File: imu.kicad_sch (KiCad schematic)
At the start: 4 parts, among them U8 MC3479

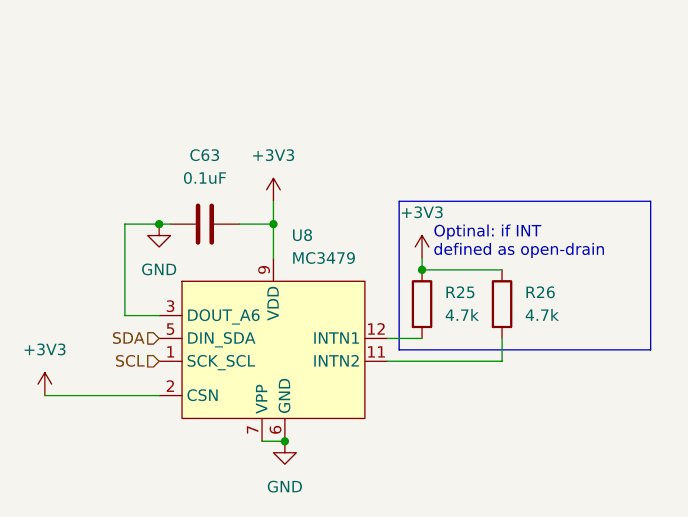
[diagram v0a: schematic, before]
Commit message: schematic creation
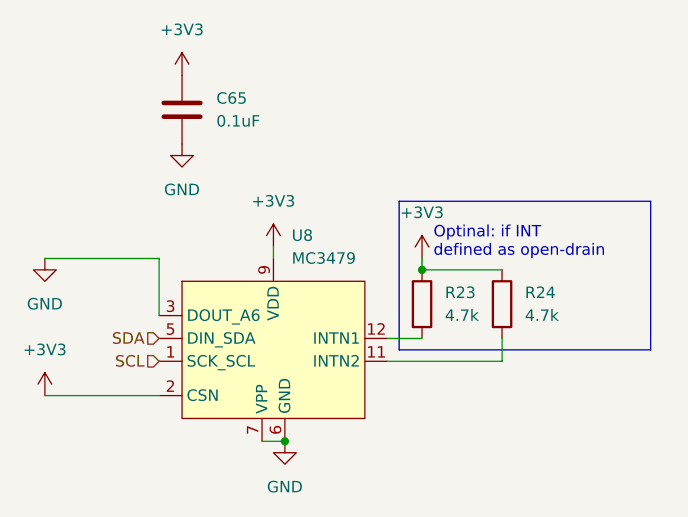
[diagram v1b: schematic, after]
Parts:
- renumbered C63 to C65, R25 to R23, R26 to R24
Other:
- moved on the sheet: C65
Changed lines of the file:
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@@
   (junction (at 157.48 88.9) (diameter 0) (color 0 0 0 0)
   )
-  (junction (at 140.97 83.82) (diameter 0) (color 0 0 0 0)
-  )
-  (junction (at 128.27 83.82) (diameter 0) (color 0 0 0 0)
-  )
   (junction (at 142.24 107.95) (diameter 0) (color 0 0 0 0)
   )
-  (wire (pts (xy 140.97 83.82) (xy 140.97 87.63))
-    (stroke (width 0) (type default) (color 0 0 0 0))
-  )
-  (wire (pts (xy 137.16 83.82) (xy 140.97 83.82))
+  (wire (pts (xy 140.97 86.36) (xy 140.97 87.63))
     (stroke (width 0) (type default) (color 0 0 0 0))
   )
@@
     (stroke (width 0) (type default) (color 0 0 0 0))
   )
-  (wire (pts (xy 124.46 83.82) (xy 128.27 83.82))
-    (stroke (width 0) (type default) (color 0 0 0 0))
-  )
-  (wire (pts (xy 124.46 93.98) (xy 124.46 83.82))
-    (stroke (width 0) (type default) (color 0 0 0 0))
-  )
   (wire (pts (xy 153.67 96.52) (xy 157.48 96.52))
     (stroke (width 0) (type default) (color 0 0 0 0))
@@
     (stroke (width 0) (type default) (color 0 0 0 0))
   )
-  (wire (pts (xy 140.97 81.28) (xy 140.97 83.82))
+  (wire (pts (xy 128.27 87.63) (xy 128.27 93.98))
     (stroke (width 0) (type default) (color 0 0 0 0))
   )
@@
     (stroke (width 0) (type default) (color 0 0 0 0))
   )
-  (wire (pts (xy 128.27 83.82) (xy 129.54 83.82))
-    (stroke (width 0) (type default) (color 0 0 0 0))
-  )
   (wire (pts (xy 139.7 107.95) (xy 142.24 107.95))
     (stroke (width 0) (type default) (color 0 0 0 0))
   )
-  (wire (pts (xy 128.27 93.98) (xy 124.46 93.98))
+  (wire (pts (xy 115.57 87.63) (xy 128.27 87.63))
     (stroke (width 0) (type default) (color 0 0 0 0))
   )
@@
     (effects (font (size 1.27 1.27)) (justify right))
   )
-  (symbol (lib_id "Device:C") (at 133.35 83.82 90) (unit 1)
-    (in_bom yes) (on_board yes) (fields_autoplaced)
-    (property "Reference" "C63" (id 0) (at 133.35 76.2 90))
-    (property "Value" "0.1uF" (id 1) (at 133.35 78.74 90))
-    (property "Footprint" "Capacitor_SMD:C_0603_1608Metric_Pad1.08x0.95mm_HandSolder" (id 2) (at 137.16 82.8548 0)
-      (effects (font (size 1.27 1.27)) hide)
-    )
-    (property "Datasheet" "~" (id 3) (at 133.35 83.82 0)
-      (effects (font (size 1.27 1.27)) hide)
-    )
-    (pin "1")
-    (pin "2")
+  (symbol (lib_id "Device:C") (at 130.81 71.12 180) (unit 1)
+    (in_bom yes) (on_board yes) (fields_autoplaced)
+    (property "Reference" "C65" (id 0) (at 134.62 69.8499 0)
+      (effects (font (size 1.27 1.27)) (justify right))
+    )
+    (property "Value" "0.1uF" (id 1) (at 134.62 72.3899 0)
+      (effects (font (size 1.27 1.27)) (justify right))
+    )
+    (property "Footprint" "Capacitor_SMD:C_0603_1608Metric_Pad1.08x0.95mm_HandSolder" (id 2) (at 129.8448 67.31 0)
+      (effects (font (size 1.27 1.27)) hide)
+    )
+    (property "Datasheet" "~" (id 3) (at 130.81 71.12 0)
+      (effects (font (size 1.27 1.27)) hide)
+    )
+    (pin "1")
+    (pin "2")
+  )
+  (symbol (lib_id "power:+3V3") (at 140.97 86.36 0) (unit 1)
+    (in_bom yes) (on_board yes) (fields_autoplaced)
+    (property "Reference" "#PWR075" (id 0) (at 140.97 90.17 0)
+      (effects (font (size 1.27 1.27)) hide)
+    )
+    (property "Value" "+3V3" (id 1) (at 140.97 81.28 0))
+    (property "Footprint" "" (id 2) (at 140.97 86.36 0)
+      (effects (font (size 1.27 1.27)) hide)
+    )
+    (property "Datasheet" "" (id 3) (at 140.97 86.36 0)
+      (effects (font (size 1.27 1.27)) hide)
+    )
+    (pin "1")
   )
   (symbol (lib_id "Device:R") (at 157.48 92.71 0) (unit 1)
     (in_bom yes) (on_board yes) (fields_autoplaced)
-    (property "Reference" "R25" (id 0) (at 160.02 91.4399 0)
+    (property "Reference" "R23" (id 0) (at 160.02 91.4399 0)
       (effects (font (size 1.27 1.27)) (justify left))
     )
@@
     (pin "2")
   )
-  (symbol (lib_id "power:+3V3") (at 140.97 81.28 0) (unit 1)
-    (in_bom yes) (on_board yes) (fields_autoplaced)
-    (property "Reference" "#PWR070" (id 0) (at 140.97 85.09 0)
-      (effects (font (size 1.27 1.27)) hide)
-    )
-    (property "Value" "+3V3" (id 1) (at 140.97 76.2 0))
-    (property "Footprint" "" (id 2) (at 140.97 81.28 0)
-      (effects (font (size 1.27 1.27)) hide)
-    )
-    (property "Datasheet" "" (id 3) (at 140.97 81.28 0)
+  (symbol (lib_id "power:+3V3") (at 130.81 67.31 0) (unit 1)
+    (in_bom yes) (on_board yes) (fields_autoplaced)
+    (property "Reference" "#PWR073" (id 0) (at 130.81 71.12 0)
+      (effects (font (size 1.27 1.27)) hide)
+    )
+    (property "Value" "+3V3" (id 1) (at 130.81 62.23 0))
+    (property "Footprint" "" (id 2) (at 130.81 67.31 0)
+      (effects (font (size 1.27 1.27)) hide)
+    )
+    (property "Datasheet" "" (id 3) (at 130.81 67.31 0)
       (effects (font (size 1.27 1.27)) hide)
     )
@@
   (symbol (lib_id "power:+3V3") (at 115.57 102.87 0) (unit 1)
     (in_bom yes) (on_board yes) (fields_autoplaced)
-    (property "Reference" "#PWR068" (id 0) (at 115.57 106.68 0)
+    (property "Reference" "#PWR072" (id 0) (at 115.57 106.68 0)
       (effects (font (size 1.27 1.27)) hide)
     )
@@
     (pin "1")
   )
+  (symbol (lib_id "power:GND") (at 115.57 87.63 0) (unit 1)
+    (in_bom yes) (on_board yes) (fields_autoplaced)
+    (property "Reference" "#PWR071" (id 0) (at 115.57 93.98 0)
+      (effects (font (size 1.27 1.27)) hide)
+    )
+    (property "Value" "GND" (id 1) (at 115.57 92.71 0))
+    (property "Footprint" "" (id 2) (at 115.57 87.63 0)
+      (effects (font (size 1.27 1.27)) hide)
+    )
+    (property "Datasheet" "" (id 3) (at 115.57 87.63 0)
+      (effects (font (size 1.27 1.27)) hide)
+    )
+    (pin "1")
+  )
   (symbol (lib_id "Device:R") (at 166.37 92.71 0) (unit 1)
     (in_bom yes) (on_board yes) (fields_autoplaced)
-    (property "Reference" "R26" (id 0) (at 168.91 91.4399 0)
+    (property "Reference" "R24" (id 0) (at 168.91 91.4399 0)
       (effects (font (size 1.27 1.27)) (justify left))
     )
@@
   (symbol (lib_id "power:+3V3") (at 157.48 87.63 0) (unit 1)
     (in_bom yes) (on_board yes) (fields_autoplaced)
-    (property "Reference" "#PWR072" (id 0) (at 157.48 91.44 0)
+    (property "Reference" "#PWR077" (id 0) (at 157.48 91.44 0)
       (effects (font (size 1.27 1.27)) hide)
     )
@@
     (pin "9")
   )
-  (symbol (lib_id "power:GND") (at 128.27 83.82 0) (unit 1)
-    (in_bom yes) (on_board yes) (fields_autoplaced)
-    (property "Reference" "#PWR069" (id 0) (at 128.27 90.17 0)
-      (effects (font (size 1.27 1.27)) hide)
-    )
-    (property "Value" "GND" (id 1) (at 128.27 88.9 0))
-    (property "Footprint" "" (id 2) (at 128.27 83.82 0)
-      (effects (font (size 1.27 1.27)) hide)
-    )
-    (property "Datasheet" "" (id 3) (at 128.27 83.82 0)
-      (effects (font (size 1.27 1.27)) hide)
-    )
-    (pin "1")
-  )
   (symbol (lib_id "power:GND") (at 142.24 107.95 0) (unit 1)
     (in_bom yes) (on_board yes) (fields_autoplaced)
-    (property "Reference" "#PWR071" (id 0) (at 142.24 114.3 0)
+    (property "Reference" "#PWR076" (id 0) (at 142.24 114.3 0)
       (effects (font (size 1.27 1.27)) hide)
     )
@@
       (effects (font (size 1.27 1.27)) hide)
     )
+    (pin "1")
+  )
+  (symbol (lib_id "power:GND") (at 130.81 74.93 0) (unit 1)
+    (in_bom yes) (on_board yes) (fields_autoplaced)
+    (property "Reference" "#PWR074" (id 0) (at 130.81 81.28 0)
+      (effects (font (size 1.27 1.27)) hide)
+    )
+    (property "Value" "GND" (id 1) (at 130.81 80.01 0))
+    (property "Footprint" "" (id 2) (at 130.81 74.93 0)
+      (effects (font (size 1.27 1.27)) hide)
+    )
+    (property "Datasheet" "" (id 3) (at 130.81 74.93 0)
+      (effects (font (size 1.27 1.27)) hide)
+    )
